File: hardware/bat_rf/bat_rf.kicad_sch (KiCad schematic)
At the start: 95 parts, among them J1 USB_C_Receptacle_PowerOnly_6P, J2 Conn_01x04, J4 Conn_01x02, Q1 NMOS, SW2 RESET, U1 TPS54331, U3 ESP8684-WROOM-02UC, U4 CS5090E

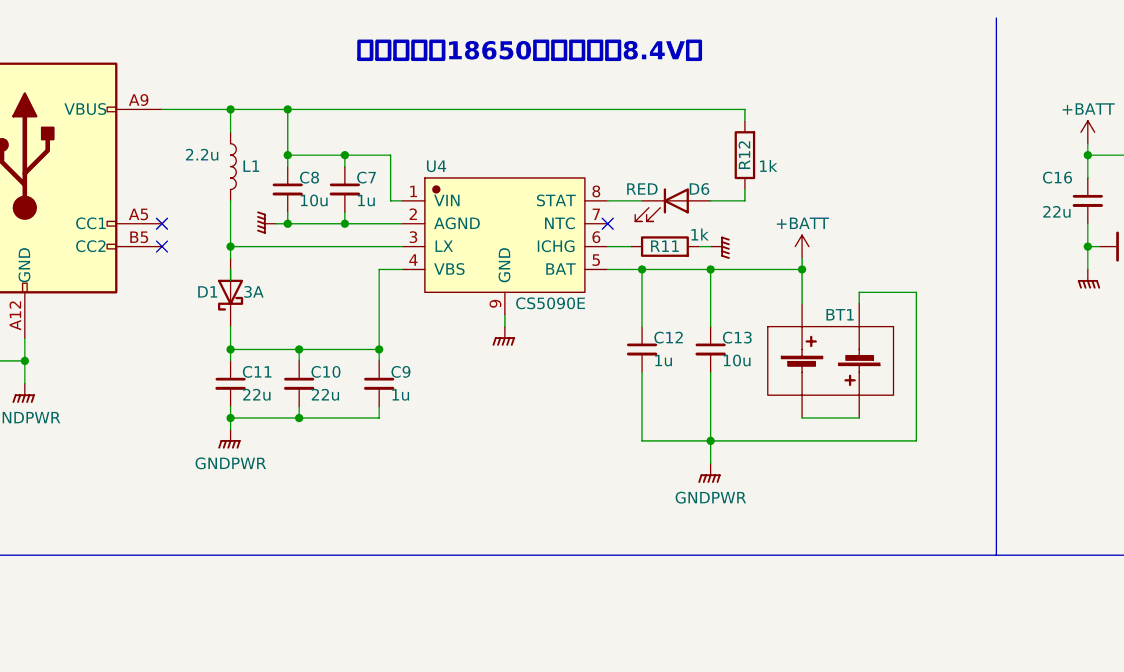
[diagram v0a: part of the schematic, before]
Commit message: 更新rfBat PCB
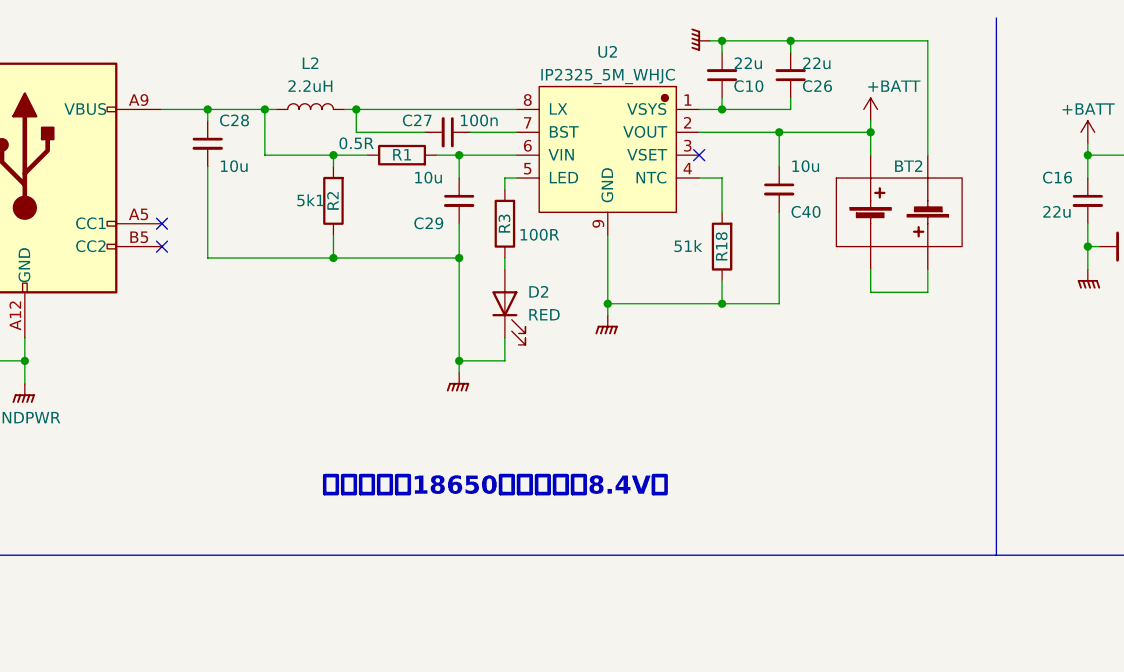
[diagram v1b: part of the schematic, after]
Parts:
- removed BT1: doubleBatCell, bat_rf:BAT-SMD_BH-18650-B1BA007, symbol bat_rf:doubleBatCell
- removed C11: 22u, Capacitor_SMD:C_0805_2012Metric_Pad1.18x1.45mm_HandSolder, symbol Device:C_Small
- removed C12, C7, C9: 1u, Capacitor_SMD:C_0603_1608Metric_Pad1.08x0.95mm_HandSolder, symbol Device:C_Small
- removed C13, C8: 10u, Capacitor_SMD:C_0805_2012Metric_Pad1.18x1.45mm_HandSolder, symbol Device:C_Small
- removed D1: 3A, Diode_SMD:D_SMA, symbol Diode:1N5711UR
- removed D6: RED, LED_SMD:LED_0603_1608Metric_Pad1.05x0.95mm_HandSolder, symbol Device:LED
- removed L1: 2.2u, bat_rf:IND-SMD_L7.0-W6.6_0630CDMCCDS, symbol Device:L
- removed R11, R12: 1k, Resistor_SMD:R_0603_1608Metric_Pad0.98x0.95mm_HandSolder, symbol Device:R
- removed U4: CS5090E, bat_rf:ESOP-8_L4.9-W3.9-P1.27-LS6.0-BL-EP, symbol bat_rf:CS5090E
- added BT2: doubleBatCell, bat_rf:BAT-SMD_BH-18650-B1BA007, symbol bat_rf:doubleBatCell
- added C26: 22u, Capacitor_SMD:C_0805_2012Metric_Pad1.18x1.45mm_HandSolder, symbol Device:C_Small
- added C27: 100n, Capacitor_SMD:C_0603_1608Metric_Pad1.08x0.95mm_HandSolder, symbol Device:C_Small
- added C28, C29, C40: 10u, Capacitor_SMD:C_0805_2012Metric_Pad1.18x1.45mm_HandSolder, symbol Device:C_Small
- added D2: RED, Capacitor_SMD:C_0805_2012Metric_Pad1.18x1.45mm_HandSolder, symbol Device:LED
- added L2: 2.2uH, Inductor_SMD_Wurth:L_Wurth_WE-LQSH-4020, symbol Device:L
- added R1: 0.5R, Resistor_SMD:R_0603_1608Metric_Pad0.98x0.95mm_HandSolder, symbol Device:R
- added R18: 51k, Resistor_SMD:R_0603_1608Metric_Pad0.98x0.95mm_HandSolder, symbol Device:R
- added R2: 5k1, Resistor_SMD:R_0603_1608Metric_Pad0.98x0.95mm_HandSolder, symbol Device:R
- added R3: 100R, Resistor_SMD:R_0603_1608Metric_Pad0.98x0.95mm_HandSolder, symbol Device:R
- added U2: IP2325_5M_WHJC, bat_rf:ESOP-8_L4.9-W3.9-P1.27-LS6.0-BL-EP3.1, symbol bat_rf:IP2325_5M_WHJC
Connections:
- net +BATT: now also BT2.1 (+), C40.1, U2.2 (VOUT)
- net GNDPWR: now also BT2.4 (-), C26.2, C28.2, C29.2, C40.2, D2.1 (K), R18.1, R2.1, U2.9 (GND)
- net at C10.1: now also C26.1, U2.1 (VSYS)
- net at J1.A9 (VBUS), J1.B9 (VBUS): now also C28.1, L2.1, R1.1, R2.2
- new net: D2.2 (A), R3.1
- new net: R3.2, U2.5 (LED)
- new net: R18.2, U2.4 (NTC)
- new net: BT2.2 (-), BT2.3 (+)
- new net: C27.1, U2.7 (BST)
- new net: C27.2, L2.2, U2.8 (LX)
- new net: C29.1, R1.2, U2.6 (VIN)
